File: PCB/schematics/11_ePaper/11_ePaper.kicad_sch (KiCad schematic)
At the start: 1 part, among them J8 Conn_01x09_Pin

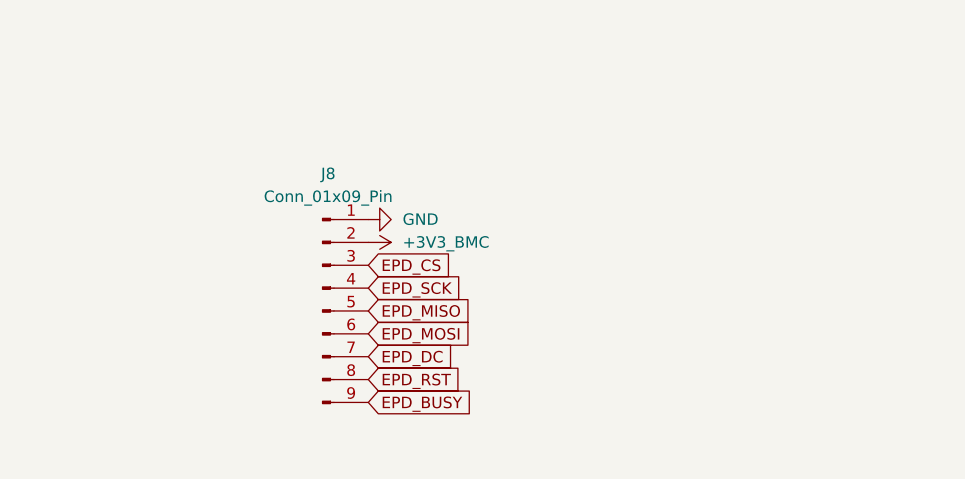
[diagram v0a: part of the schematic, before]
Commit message: Refactor : Repo
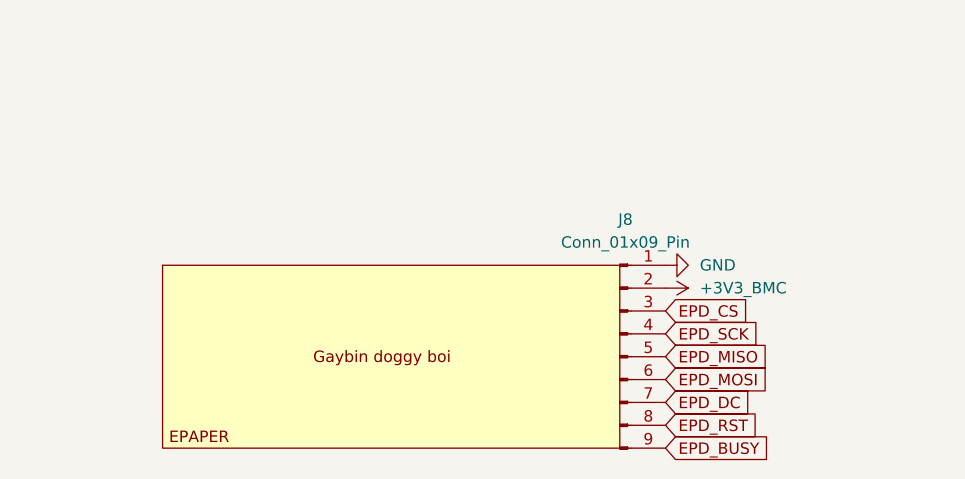
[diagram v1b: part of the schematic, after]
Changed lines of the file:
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@@
 		(stroke
 			(width 0)
-			(type default)
+			(type solid)
 		)
 		(fill
-			(type none)
+			(type color)
+			(color 255 229 191 1)
 		)
 	)
@@
 	(global_label "EPD_DC"
 		(shape input)
-		(at 91.44 77.47 0)
-		(fields_autoplaced yes)
-		(effects
-			(font
-				(size 1.27 1.27)
-			)
-			(justify left)
-		)
-		(property "Intersheetrefs" "${INTERSHEET_REFS}"
-			(at 101.6218 77.47 0)
+		(at 124.46 82.55 0)
+		(fields_autoplaced yes)
+		(effects
+			(font
+				(size 1.27 1.27)
+			)
+			(justify left)
+		)
+		(property "Intersheetrefs" "${INTERSHEET_REFS}"
+			(at 134.6418 82.55 0)
 			(hide yes)
 			(show_name no)
@@
 	(global_label "EPD_MISO"
 		(shape input)
-		(at 91.44 72.39 0)
-		(fields_autoplaced yes)
-		(effects
-			(font
-				(size 1.27 1.27)
-			)
-			(justify left)
-		)
-		(property "Intersheetrefs" "${INTERSHEET_REFS}"
-			(at 103.678 72.39 0)
+		(at 124.46 77.47 0)
+		(fields_autoplaced yes)
+		(effects
+			(font
+				(size 1.27 1.27)
+			)
+			(justify left)
+		)
+		(property "Intersheetrefs" "${INTERSHEET_REFS}"
+			(at 136.698 77.47 0)
 			(hide yes)
 			(show_name no)
@@
 	(global_label "EPD_CS"
 		(shape input)
-		(at 91.44 67.31 0)
-		(fields_autoplaced yes)
-		(effects
-			(font
-				(size 1.27 1.27)
-			)
-			(justify left)
-		)
-		(property "Intersheetrefs" "${INTERSHEET_REFS}"
-			(at 101.5613 67.31 0)
+		(at 124.46 72.39 0)
+		(fields_autoplaced yes)
+		(effects
+			(font
+				(size 1.27 1.27)
+			)
+			(justify left)
+		)
+		(property "Intersheetrefs" "${INTERSHEET_REFS}"
+			(at 134.5813 72.39 0)
 			(hide yes)
 			(show_name no)
@@
 	(global_label "EPD_SCK"
 		(shape input)
-		(at 91.44 69.85 0)
-		(fields_autoplaced yes)
-		(effects
-			(font
-				(size 1.27 1.27)
-			)
-			(justify left)
-		)
-		(property "Intersheetrefs" "${INTERSHEET_REFS}"
-			(at 102.8313 69.85 0)
+		(at 124.46 74.93 0)
+		(fields_autoplaced yes)
+		(effects
+			(font
+				(size 1.27 1.27)
+			)
+			(justify left)
+		)
+		(property "Intersheetrefs" "${INTERSHEET_REFS}"
+			(at 135.8513 74.93 0)
 			(hide yes)
 			(show_name no)
@@
 	(global_label "EPD_MOSI"
 		(shape input)
-		(at 91.44 74.93 0)
-		(fields_autoplaced yes)
-		(effects
-			(font
-				(size 1.27 1.27)
-			)
-			(justify left)
-		)
-		(property "Intersheetrefs" "${INTERSHEET_REFS}"
-			(at 103.678 74.93 0)
+		(at 124.46 80.01 0)
+		(fields_autoplaced yes)
+		(effects
+			(font
+				(size 1.27 1.27)
+			)
+			(justify left)
+		)
+		(property "Intersheetrefs" "${INTERSHEET_REFS}"
+			(at 136.698 80.01 0)
 			(hide yes)
 			(show_name no)
@@
 	(global_label "EPD_BUSY"
 		(shape input)
-		(at 91.44 82.55 0)
-		(fields_autoplaced yes)
-		(effects
-			(font
-				(size 1.27 1.27)
-			)
-			(justify left)
-		)
-		(property "Intersheetrefs" "${INTERSHEET_REFS}"
-			(at 103.9804 82.55 0)
+		(at 124.46 87.63 0)
+		(fields_autoplaced yes)
+		(effects
+			(font
+				(size 1.27 1.27)
+			)
+			(justify left)
+		)
+		(property "Intersheetrefs" "${INTERSHEET_REFS}"
+			(at 137.0004 87.63 0)
 			(hide yes)
 			(show_name no)
@@
 	(global_label "EPD_RST"
 		(shape input)
-		(at 91.44 80.01 0)
-		(fields_autoplaced yes)
-		(effects
-			(font
-				(size 1.27 1.27)
-			)
-			(justify left)
-		)
-		(property "Intersheetrefs" "${INTERSHEET_REFS}"
-			(at 102.5289 80.01 0)
+		(at 124.46 85.09 0)
+		(fields_autoplaced yes)
+		(effects
+			(font
+				(size 1.27 1.27)
+			)
+			(justify left)
+		)
+		(property "Intersheetrefs" "${INTERSHEET_REFS}"
+			(at 135.5489 85.09 0)
 			(hide yes)
 			(show_name no)
@@
 	(symbol
 		(lib_id "Connector:Conn_01x09_Pin")
-		(at 86.36 72.39 0)
+		(at 119.38 77.47 0)
 		(unit 1)
 		(body_style 1)
@@
 		(fields_autoplaced yes)
 		(property "Reference" "J8"
-			(at 86.995 57.15 0)
+			(at 120.015 62.23 0)
 			(show_name no)
 			(do_not_autoplace no)
@@
 		)
 		(property "Value" "Conn_01x09_Pin"
-			(at 86.995 59.69 0)
+			(at 120.015 64.77 0)
 			(show_name no)
 			(do_not_autoplace no)
@@
 		)
 		(property "Footprint" "Connector_PinHeader_2.54mm:PinHeader_1x09_P2.54mm_Vertical"
-			(at 86.36 72.39 0)
+			(at 99.568 90.17 0)
 			(hide yes)
 			(show_name no)
@@
 		)
 		(property "Datasheet" ""
-			(at 86.36 72.39 0)
+			(at 119.38 77.47 0)
 			(hide yes)
 			(show_name no)
@@
 		)
 		(property "Description" "Generic connector, single row, 01x09, script generated"
-			(at 86.36 72.39 0)
+			(at 98.552 90.678 0)
 			(hide yes)
 			(show_name no)
@@
 	(symbol
 		(lib_id "power:GND")
-		(at 91.44 62.23 90)
+		(at 124.46 67.31 90)
 		(unit 1)
 		(body_style 1)
@@
 		(fields_autoplaced yes)
 		(property "Reference" "#PWR01202"
-			(at 97.79 62.23 0)
+			(at 130.81 67.31 0)
 			(hide yes)
 			(show_name no)
@@
 		)
 		(property "Value" "GND"
-			(at 95.25 62.2299 90)
+			(at 128.27 67.3099 90)
 			(show_name no)
 			(do_not_autoplace no)
@@
 		)
 		(property "Footprint" ""
-			(at 91.44 62.23 0)
+			(at 124.46 67.31 0)
 			(hide yes)
 			(show_name no)
@@
 		)
 		(property "Datasheet" ""
-			(at 91.44 62.23 0)
+			(at 124.46 67.31 0)
 			(hide yes)
 			(show_name no)
@@
 		)
 		(property "Description" "Power symbol creates a global label with name \"GND\" , ground"
-			(at 91.44 62.23 0)
+			(at 124.46 67.31 0)
 			(hide yes)
 			(show_name no)
@@
 	(symbol
 		(lib_id "power:+3V3")
-		(at 91.44 64.77 270)
+		(at 124.46 69.85 270)
 		(unit 1)
 		(body_style 1)
@@
 		(fields_autoplaced yes)
 		(property "Reference" "#PWR01203"
-			(at 87.63 64.77 0)
+			(at 120.65 69.85 0)
 			(hide yes)
 			(show_name no)
@@
 		)
 		(property "Value" "+3V3_BMC"
-			(at 95.25 64.7699 90)
+			(at 128.27 69.8499 90)
 			(show_name no)
 			(do_not_autoplace no)
@@
 		)
 		(property "Footprint" ""
-			(at 91.44 64.77 0)
+			(at 124.46 69.85 0)
 			(hide yes)
 			(show_name no)
@@
 		)
 		(property "Datasheet" ""
-			(at 91.44 64.77 0)
+			(at 124.46 69.85 0)
 			(hide yes)
 			(show_name no)
@@
 		)
 		(property "Description" "Power symbol creates a global label with name \"+3V3\""
-			(at 91.44 64.77 0)
-			(hide yes)
-			(show_name no)
+			(at 124.46 69.85 0)
+			(hide yes)
+			(show_name no)
